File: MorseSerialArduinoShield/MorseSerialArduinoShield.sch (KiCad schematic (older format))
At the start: 12 parts, among them U1 SC39-11SRWA

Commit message: pre pcb design
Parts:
- BZ1: footprint (none) -> Buzzer_Beeper:Buzzer_15x7.5RM7.6
- R1, R2, R3, R4, R5, R6, R7, R8: footprint (none) -> Resistor_THT:R_Axial_DIN0309_L9.0mm_D3.2mm_P12.70mm_Horizontal
- RV1: footprint (none) -> Potentiometer_THT:Potentiometer_Piher_PT-15-V15_Vertical
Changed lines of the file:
@@
 F 0 "BZ1" H 4902 1479 50  0000 L CNN
 F 1 "Buzzer" H 4902 1388 50  0000 L CNN
-F 2 "" V 4725 1550 50  0001 C CNN
+F 2 "Buzzer_Beeper:Buzzer_15x7.5RM7.6" V 4725 1550 50  0001 C CNN
 F 3 "~" V 4725 1550 50  0001 C CNN
 	1    4750 1450
@@
 F 0 "R8" H 4920 2746 50  0000 L CNN
 F 1 "1K" H 4920 2655 50  0000 L CNN
-F 2 "" V 4780 2700 50  0001 C CNN
+F 2 "Resistor_THT:R_Axial_DIN0309_L9.0mm_D3.2mm_P12.70mm_Horizontal" V 4780 2700 50  0001 C CNN
 F 3 "~" H 4850 2700 50  0001 C CNN
 	1    4850 2700
@@
 F 0 "R7" H 4920 2646 50  0000 L CNN
 F 1 "1K" H 4920 2555 50  0000 L CNN
-F 2 "" V 4780 2600 50  0001 C CNN
+F 2 "Resistor_THT:R_Axial_DIN0309_L9.0mm_D3.2mm_P12.70mm_Horizontal" V 4780 2600 50  0001 C CNN
 F 3 "~" H 4850 2600 50  0001 C CNN
 	1    4850 2600
@@
 F 0 "R6" H 4920 2546 50  0000 L CNN
 F 1 "1K" H 4920 2455 50  0000 L CNN
-F 2 "" V 4780 2500 50  0001 C CNN
+F 2 "Resistor_THT:R_Axial_DIN0309_L9.0mm_D3.2mm_P12.70mm_Horizontal" V 4780 2500 50  0001 C CNN
 F 3 "~" H 4850 2500 50  0001 C CNN
 	1    4850 2500
@@
 F 0 "R5" H 4920 2446 50  0000 L CNN
 F 1 "1K" H 4920 2355 50  0000 L CNN
-F 2 "" V 4780 2400 50  0001 C CNN
+F 2 "Resistor_THT:R_Axial_DIN0309_L9.0mm_D3.2mm_P12.70mm_Horizontal" V 4780 2400 50  0001 C CNN
 F 3 "~" H 4850 2400 50  0001 C CNN
 	1    4850 2400
@@
 F 0 "R4" H 4920 2346 50  0000 L CNN
 F 1 "1K" H 4920 2255 50  0000 L CNN
-F 2 "" V 4780 2300 50  0001 C CNN
+F 2 "Resistor_THT:R_Axial_DIN0309_L9.0mm_D3.2mm_P12.70mm_Horizontal" V 4780 2300 50  0001 C CNN
 F 3 "~" H 4850 2300 50  0001 C CNN
 	1    4850 2300
@@
 F 0 "R3" H 4920 2246 50  0000 L CNN
 F 1 "1K" H 4920 2155 50  0000 L CNN
-F 2 "" V 4780 2200 50  0001 C CNN
+F 2 "Resistor_THT:R_Axial_DIN0309_L9.0mm_D3.2mm_P12.70mm_Horizontal" V 4780 2200 50  0001 C CNN
 F 3 "~" H 4850 2200 50  0001 C CNN
 	1    4850 2200
@@
 F 0 "R2" H 4920 2146 50  0000 L CNN
 F 1 "1K" H 4920 2055 50  0000 L CNN
-F 2 "" V 4780 2100 50  0001 C CNN
+F 2 "Resistor_THT:R_Axial_DIN0309_L9.0mm_D3.2mm_P12.70mm_Horizontal" V 4780 2100 50  0001 C CNN
 F 3 "~" H 4850 2100 50  0001 C CNN
 	1    4850 2100
@@
 F 0 "RV1" H 4030 1596 50  0000 R CNN
 F 1 "R_POT_TRIM" H 4030 1505 50  0000 R CNN
-F 2 "" H 4100 1550 50  0001 C CNN
+F 2 "Potentiometer_THT:Potentiometer_Piher_PT-15-V15_Vertical" H 4100 1550 50  0001 C CNN
 F 3 "~" H 4100 1550 50  0001 C CNN
 	1    4100 1550
@@
 F 0 "R1" H 4920 2046 50  0000 L CNN
 F 1 "1K" H 4920 1955 50  0000 L CNN
-F 2 "" V 4780 2000 50  0001 C CNN
+F 2 "Resistor_THT:R_Axial_DIN0309_L9.0mm_D3.2mm_P12.70mm_Horizontal" V 4780 2000 50  0001 C CNN
 F 3 "~" H 4850 2000 50  0001 C CNN
 	1    4850 2000

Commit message: BaseLine PCB design
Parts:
- RV1: footprint Potentiometer_THT:Potentiometer_Piher_PT-15-V15_Vertical -> Potentiometer_THT:Potentiometer_Runtron_RM-065_Vertical
- U1: footprint Display_7Segment:Sx39-1xxxxx -> Display_7Segment:7SegmentLED_LTS6760_LTS6780
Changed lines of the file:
@@
 F 0 "RV1" H 4030 1596 50  0000 R CNN
 F 1 "R_POT_TRIM" H 4030 1505 50  0000 R CNN
-F 2 "Potentiometer_THT:Potentiometer_Piher_PT-15-V15_Vertical" H 4100 1550 50  0001 C CNN
+F 2 "Potentiometer_THT:Potentiometer_Runtron_RM-065_Vertical" H 4100 1550 50  0001 C CNN
 F 3 "~" H 4100 1550 50  0001 C CNN
 	1    4100 1550
@@
 F 0 "U1" H 5300 2967 50  0000 C CNN
 F 1 "SC39-11SRWA" H 5300 2876 50  0000 C CNN
-F 2 "Display_7Segment:Sx39-1xxxxx" H 5300 1750 50  0001 C CNN
+F 2 "Display_7Segment:7SegmentLED_LTS6760_LTS6780" H 5300 1750 50  0001 C CNN
 F 3 "http://www.kingbrightusa.com/images/catalog/SPEC/sc39-11srwa.pdf" H 5300 2300 50  0001 C CNN
 	1    5300 2300

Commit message: startpoint
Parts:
- BZ1: footprint Buzzer_Beeper:Buzzer_15x7.5RM7.6 -> Buzzer_Beeper:Buzzer_12x9.5RM7.6
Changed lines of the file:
@@
 F 0 "BZ1" H 4902 1479 50  0000 L CNN
 F 1 "Buzzer" H 4902 1388 50  0000 L CNN
-F 2 "Buzzer_Beeper:Buzzer_15x7.5RM7.6" V 4725 1550 50  0001 C CNN
+F 2 "Buzzer_Beeper:Buzzer_12x9.5RM7.6" V 4725 1550 50  0001 C CNN
 F 3 "~" V 4725 1550 50  0001 C CNN
 	1    4750 1450

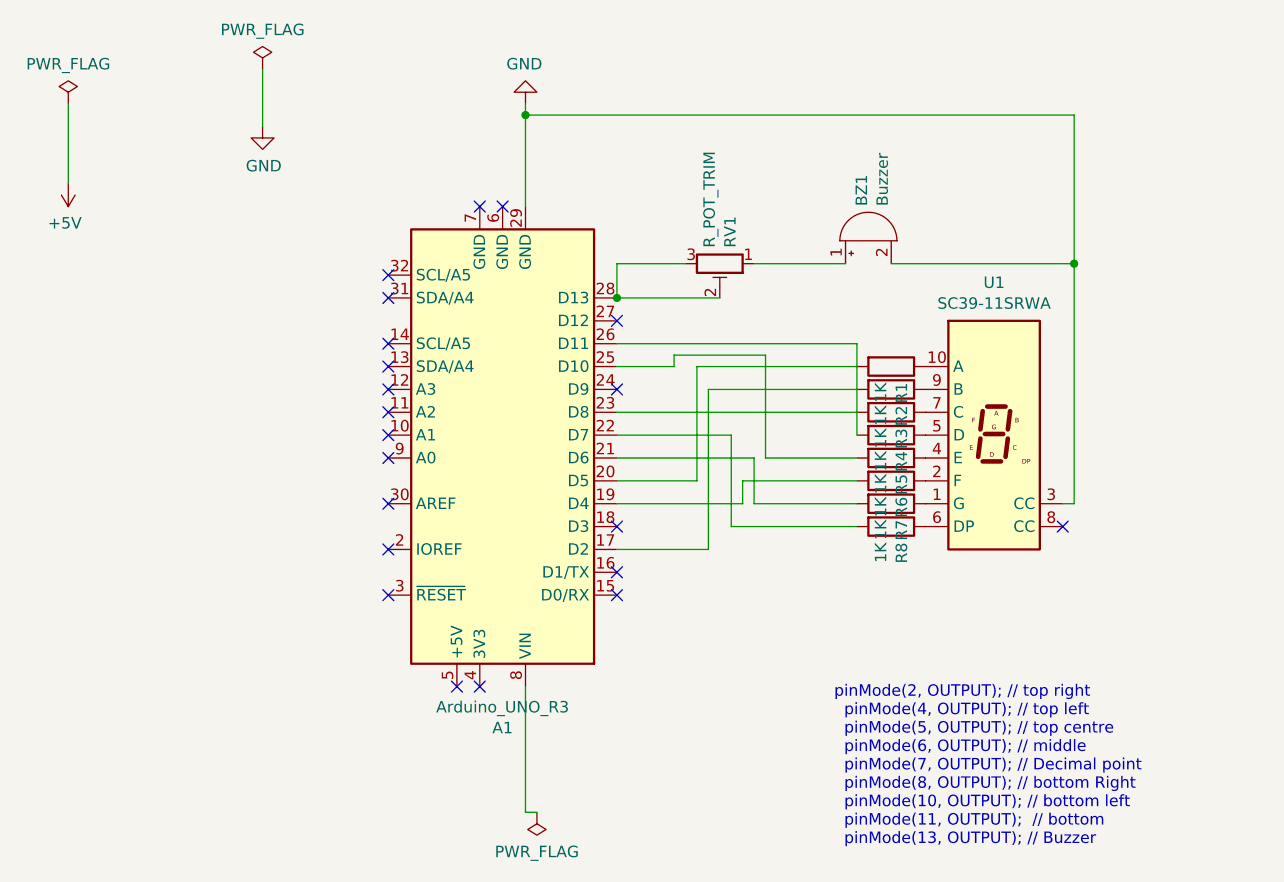
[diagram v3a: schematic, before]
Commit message: fright hand rework
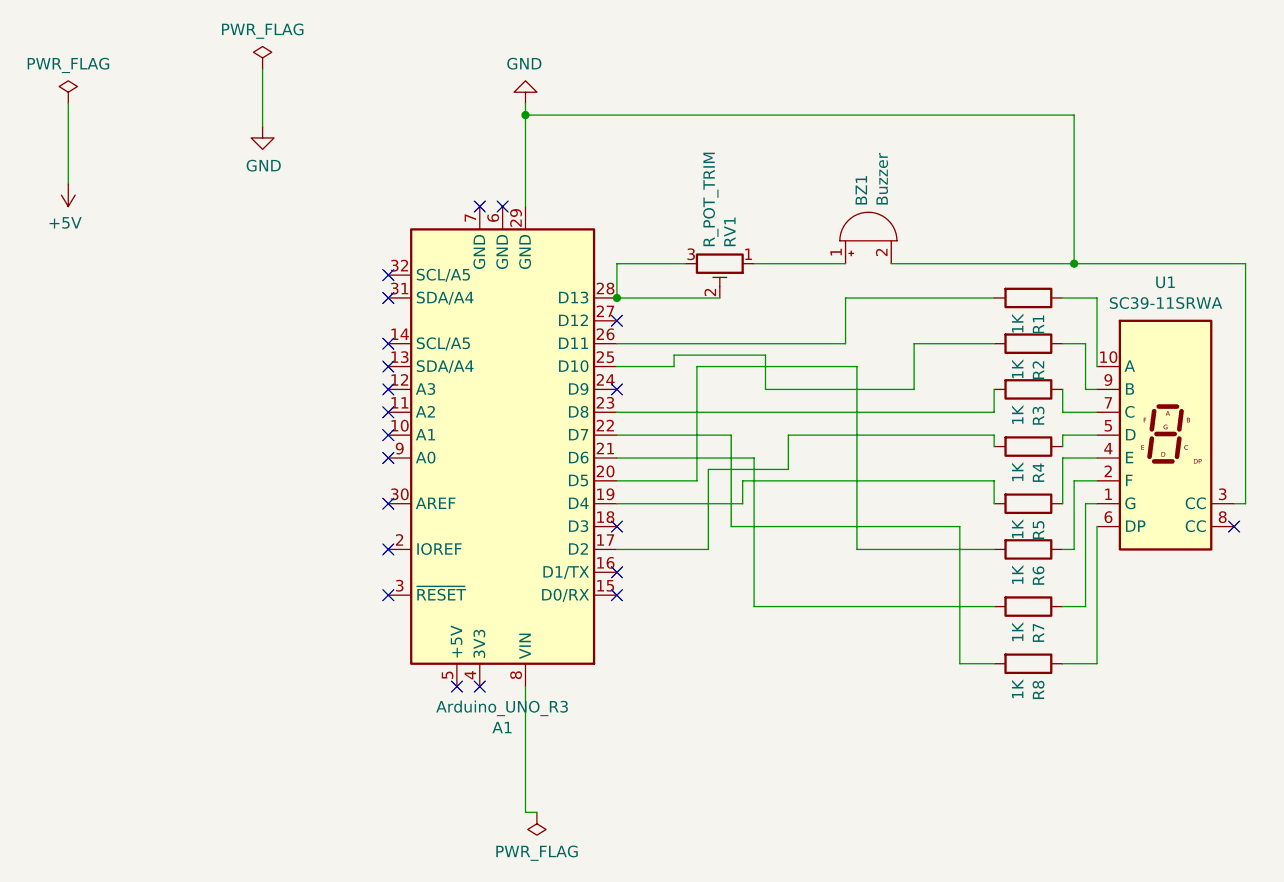
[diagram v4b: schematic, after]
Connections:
- net at A1.17 (D2): now also R4.2; no longer R2.2
- net at A1.19 (D4): now also R5.2; no longer R6.2
- net at A1.20 (D5): now also R6.2; no longer R1.2
- net at A1.25 (D10): now also R2.2; no longer R5.2
- net at A1.26 (D11): now also R1.2; no longer R4.2
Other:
- note removed: "pinMode(2, OUTPUT); // top right\n pinMode(4, OUTPUT); // top left\n pinMode(5, OUTPUT); // top centre\n pinMode(6, OUTPUT); // middle\n pinMode(7, OUTPUT); // Decimal point\n pinMode(8, OUTPUT); // bottom Right\n pinMode(10, OUTPUT); // bottom left\n pinMode(11, OUTPUT); // bottom\n pinMode(13, OUTPUT); // Buzzer"
- moved on the sheet: R1, R2, R3, R4, R5, R6, R7, R8, U1
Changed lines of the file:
@@
 L Device:R R8
 U 1 1 5E8A1C48
-P 4850 2700
-F 0 "R8" H 4920 2746 50  0000 L CNN
-F 1 "1K" H 4920 2655 50  0000 L CNN
-F 2 "Resistor_THT:R_Axial_DIN0309_L9.0mm_D3.2mm_P12.70mm_Horizontal" V 4780 2700 50  0001 C CNN
-F 3 "~" H 4850 2700 50  0001 C CNN
-	1    4850 2700
+P 5450 3300
+F 0 "R8" H 5520 3346 50  0000 L CNN
+F 1 "1K" H 5520 3255 50  0000 L CNN
+F 2 "Resistor_THT:R_Axial_DIN0309_L9.0mm_D3.2mm_P12.70mm_Horizontal" V 5380 3300 50  0001 C CNN
+F 3 "~" H 5450 3300 50  0001 C CNN
+	1    5450 3300
 	0    1    1    0
 $EndComp
@@
 L Device:R R7
 U 1 1 5ECADC31
-P 4850 2600
-F 0 "R7" H 4920 2646 50  0000 L CNN
-F 1 "1K" H 4920 2555 50  0000 L CNN
-F 2 "Resistor_THT:R_Axial_DIN0309_L9.0mm_D3.2mm_P12.70mm_Horizontal" V 4780 2600 50  0001 C CNN
-F 3 "~" H 4850 2600 50  0001 C CNN
-	1    4850 2600
+P 5450 3050
+F 0 "R7" H 5520 3096 50  0000 L CNN
+F 1 "1K" H 5520 3005 50  0000 L CNN
+F 2 "Resistor_THT:R_Axial_DIN0309_L9.0mm_D3.2mm_P12.70mm_Horizontal" V 5380 3050 50  0001 C CNN
+F 3 "~" H 5450 3050 50  0001 C CNN
+	1    5450 3050
 	0    1    1    0
 $EndComp
@@
 L Device:R R6
 U 1 1 5ECAE2EE
-P 4850 2500
-F 0 "R6" H 4920 2546 50  0000 L CNN
-F 1 "1K" H 4920 2455 50  0000 L CNN
-F 2 "Resistor_THT:R_Axial_DIN0309_L9.0mm_D3.2mm_P12.70mm_Horizontal" V 4780 2500 50  0001 C CNN
-F 3 "~" H 4850 2500 50  0001 C CNN
-	1    4850 2500
+P 5450 2800
+F 0 "R6" H 5520 2846 50  0000 L CNN
+F 1 "1K" H 5520 2755 50  0000 L CNN
+F 2 "Resistor_THT:R_Axial_DIN0309_L9.0mm_D3.2mm_P12.70mm_Horizontal" V 5380 2800 50  0001 C CNN
+F 3 "~" H 5450 2800 50  0001 C CNN
+	1    5450 2800
 	0    1    1    0
 $EndComp
@@
 L Device:R R5
 U 1 1 5ECAE473
-P 4850 2400
-F 0 "R5" H 4920 2446 50  0000 L CNN
-F 1 "1K" H 4920 2355 50  0000 L CNN
-F 2 "Resistor_THT:R_Axial_DIN0309_L9.0mm_D3.2mm_P12.70mm_Horizontal" V 4780 2400 50  0001 C CNN
-F 3 "~" H 4850 2400 50  0001 C CNN
-	1    4850 2400
+P 5450 2600
+F 0 "R5" H 5520 2646 50  0000 L CNN
+F 1 "1K" H 5520 2555 50  0000 L CNN
+F 2 "Resistor_THT:R_Axial_DIN0309_L9.0mm_D3.2mm_P12.70mm_Horizontal" V 5380 2600 50  0001 C CNN
+F 3 "~" H 5450 2600 50  0001 C CNN
+	1    5450 2600
 	0    1    1    0
 $EndComp
@@
 L Device:R R4
 U 1 1 5ECAE650
-P 4850 2300
-F 0 "R4" H 4920 2346 50  0000 L CNN
-F 1 "1K" H 4920 2255 50  0000 L CNN
-F 2 "Resistor_THT:R_Axial_DIN0309_L9.0mm_D3.2mm_P12.70mm_Horizontal" V 4780 2300 50  0001 C CNN
-F 3 "~" H 4850 2300 50  0001 C CNN
-	1    4850 2300
+P 5450 2350
+F 0 "R4" H 5520 2396 50  0000 L CNN
+F 1 "1K" H 5520 2305 50  0000 L CNN
+F 2 "Resistor_THT:R_Axial_DIN0309_L9.0mm_D3.2mm_P12.70mm_Horizontal" V 5380 2350 50  0001 C CNN
+F 3 "~" H 5450 2350 50  0001 C CNN
+	1    5450 2350
 	0    1    1    0
 $EndComp
@@
 L Device:R R3
 U 1 1 5ECAE844
-P 4850 2200
-F 0 "R3" H 4920 2246 50  0000 L CNN
-F 1 "1K" H 4920 2155 50  0000 L CNN
-F 2 "Resistor_THT:R_Axial_DIN0309_L9.0mm_D3.2mm_P12.70mm_Horizontal" V 4780 2200 50  0001 C CNN
-F 3 "~" H 4850 2200 50  0001 C CNN
-	1    4850 2200
+P 5450 2100
+F 0 "R3" H 5520 2146 50  0000 L CNN
+F 1 "1K" H 5520 2055 50  0000 L CNN
+F 2 "Resistor_THT:R_Axial_DIN0309_L9.0mm_D3.2mm_P12.70mm_Horizontal" V 5380 2100 50  0001 C CNN
+F 3 "~" H 5450 2100 50  0001 C CNN
+	1    5450 2100
 	0    1    1    0
 $EndComp
@@
 L Device:R R2
 U 1 1 5ECAEC2F
-P 4850 2100
-F 0 "R2" H 4920 2146 50  0000 L CNN
-F 1 "1K" H 4920 2055 50  0000 L CNN
-F 2 "Resistor_THT:R_Axial_DIN0309_L9.0mm_D3.2mm_P12.70mm_Horizontal" V 4780 2100 50  0001 C CNN
-F 3 "~" H 4850 2100 50  0001 C CNN
-	1    4850 2100
-	0    1    1    0
-$EndComp
-Text Notes 4600 4100 0    50   ~ 0
-  pinMode(2, OUTPUT); // top right\n  pinMode(4, OUTPUT); // top left\n  pinMode(5, OUTPUT); // top centre\n  pinMode(6, OUTPUT); // middle\n  pinMode(7, OUTPUT); // Decimal point\n  pinMode(8, OUTPUT); // bottom Right\n  pinMode(10, OUTPUT); // bottom left\n  pinMode(11, OUTPUT);  // bottom\n  pinMode(13, OUTPUT); // Buzzer
+P 5450 1900
+F 0 "R2" H 5520 1946 50  0000 L CNN
+F 1 "1K" H 5520 1855 50  0000 L CNN
+F 2 "Resistor_THT:R_Axial_DIN0309_L9.0mm_D3.2mm_P12.70mm_Horizontal" V 5380 1900 50  0001 C CNN
+F 3 "~" H 5450 1900 50  0001 C CNN
+	1    5450 1900
+	0    1    1    0
+$EndComp
 $Comp
 L MCU_Module:Arduino_UNO_R3 A1
@@
 	4850 1550 5650 1550
 Wire Wire Line
-	4050 2800 4050 2100
-Wire Wire Line
-	4050 2100 4700 2100
-Wire Wire Line
-	3650 2800 4050 2800
-Wire Wire Line
-	4200 2500 4700 2500
-Wire Wire Line
 	3650 2500 4000 2500
 Wire Wire Line
@@
 	3650 2400 4250 2400
 Wire Wire Line
-	4250 2400 4250 2600
-Wire Wire Line
-	4250 2600 4700 2600
-Wire Wire Line
 	4200 2600 4200 2500
 Wire Wire Line
@@
 	4150 2300 4150 2700
 Wire Wire Line
-	4150 2700 4700 2700
-Wire Wire Line
-	3650 2200 4700 2200
-Wire Wire Line
 	4000 2000 4700 2000
 Wire Wire Line
@@
 Wire Wire Line
 	3900 1950 4300 1950
-Wire Wire Line
-	4300 1950 4300 2400
-Wire Wire Line
-	4300 2400 4700 2400
-Wire Wire Line
-	3650 1900 4700 1900
-Wire Wire Line
-	4700 1900 4700 2300
 $Comp
 L Device:R R1
 U 1 1 5ECAEFA7
-P 4850 2000
-F 0 "R1" H 4920 2046 50  0000 L CNN
-F 1 "1K" H 4920 1955 50  0000 L CNN
-F 2 "Resistor_THT:R_Axial_DIN0309_L9.0mm_D3.2mm_P12.70mm_Horizontal" V 4780 2000 50  0001 C CNN
-F 3 "~" H 4850 2000 50  0001 C CNN
-	1    4850 2000
+P 5450 1700
+F 0 "R1" H 5520 1746 50  0000 L CNN
+F 1 "1K" H 5520 1655 50  0000 L CNN
+F 2 "Resistor_THT:R_Axial_DIN0309_L9.0mm_D3.2mm_P12.70mm_Horizontal" V 5380 1700 50  0001 C CNN
+F 3 "~" H 5450 1700 50  0001 C CNN
+	1    5450 1700
 	0    1    1    0
 $EndComp
@@
 L Display_Character:SC39-11SRWA U1
 U 1 1 5E8A0889
-P 5300 2300
-F 0 "U1" H 5300 2967 50  0000 C CNN
-F 1 "SC39-11SRWA" H 5300 2876 50  0000 C CNN
-F 2 "Display_7Segment:7SegmentLED_LTS6760_LTS6780" H 5300 1750 50  0001 C CNN
-F 3 "http://www.kingbrightusa.com/images/catalog/SPEC/sc39-11srwa.pdf" H 5300 2300 50  0001 C CNN
-	1    5300 2300
+P 6050 2300
+F 0 "U1" H 6050 2967 50  0000 C CNN
+F 1 "SC39-11SRWA" H 6050 2876 50  0000 C CNN
+F 2 "Display_7Segment:7SegmentLED_LTS6760_LTS6780" H 6050 1750 50  0001 C CNN
+F 3 "http://www.kingbrightusa.com/images/catalog/SPEC/sc39-11srwa.pdf" H 6050 2300 50  0001 C CNN
+	1    6050 2300
 	1    0    0    -1
 $EndComp
 Wire Wire Line
-	5650 1550 5650 2600
-Wire Wire Line
-	5650 2600 5600 2600
-Connection ~ 5650 1550
-NoConn ~ 5600 2700
+	6400 2600 6350 2600
+NoConn ~ 6350 2700
 NoConn ~ 3650 3000
 NoConn ~ 3650 2900
@@
 	3250 850  3250 900
 Connection ~ 3250 900
+Wire Wire Line
+	3650 2800 4050 2800
+Wire Wire Line
+	4300 1950 4300 2100
+Wire Wire Line
+	4050 2450 4050 2800
+Wire Wire Line
+	4050 2450 4400 2450
+Wire Wire Line
+	5650 1550 6400 1550
+Wire Wire Line
+	6400 1550 6400 2600
+Connection ~ 5650 1550
+Wire Wire Line
+	4950 2100 4950 1900
+Wire Wire Line
+	4950 1900 5300 1900
+Wire Wire Line
+	4300 2100 4950 2100
+Wire Wire Line
+	5300 2200 5300 2100
+Wire Wire Line
+	3650 2200 5300 2200
+Wire Wire Line
+	5150 2700 5150 3300
+Wire Wire Line
+	5150 3300 5300 3300
+Wire Wire Line
+	4150 2700 5150 2700
+Wire Wire Line
+	5600 1700 5750 1700
+Wire Wire Line
+	5750 1700 5750 2000
+Wire Wire Line
+	5600 1900 5700 1900
+Wire Wire Line
+	5700 1900 5700 2100
+Wire Wire Line
+	5700 2100 5750 2100
+Wire Wire Line
+	5600 2100 5600 2200
+Wire Wire Line
+	5600 2200 5750 2200
+Wire Wire Line
+	5600 2350 5600 2300
+Wire Wire Line
+	5600 2300 5750 2300
+Wire Wire Line
+	5600 2600 5600 2400
+Wire Wire Line
+	5600 2400 5750 2400
+Wire Wire Line
+	5600 2800 5650 2800
+Wire Wire Line
+	5650 2800 5650 2500
+Wire Wire Line
+	5650 2500 5750 2500
+Wire Wire Line
+	5600 3050 5700 3050
+Wire Wire Line
+	5700 3050 5700 2600
+Wire Wire Line
+	5700 2600 5750 2600
+Wire Wire Line
+	5600 3300 5750 3300
+Wire Wire Line
+	5750 3300 5750 2700
+Wire Wire Line
+	4400 2450 4400 2300
+Wire Wire Line
+	4400 2300 5300 2300
+Wire Wire Line
+	5300 2300 5300 2350
+Wire Wire Line
+	4650 1900 4650 1700
+Wire Wire Line
+	4650 1700 5300 1700
+Wire Wire Line
+	3650 1900 4650 1900
+Wire Wire Line
+	5300 2500 5300 2600
+Wire Wire Line
+	4200 2500 5300 2500
+Wire Wire Line
+	4700 2000 4700 2800
+Wire Wire Line
+	4700 2800 5300 2800
+Wire Wire Line
+	4250 3050 5300 3050
+Wire Wire Line
+	4250 2400 4250 3050
 $EndSCHEMATC
